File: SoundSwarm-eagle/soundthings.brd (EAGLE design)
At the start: 100 x 40 mm, 33 parts, among them Q2 IRLB8721PBF

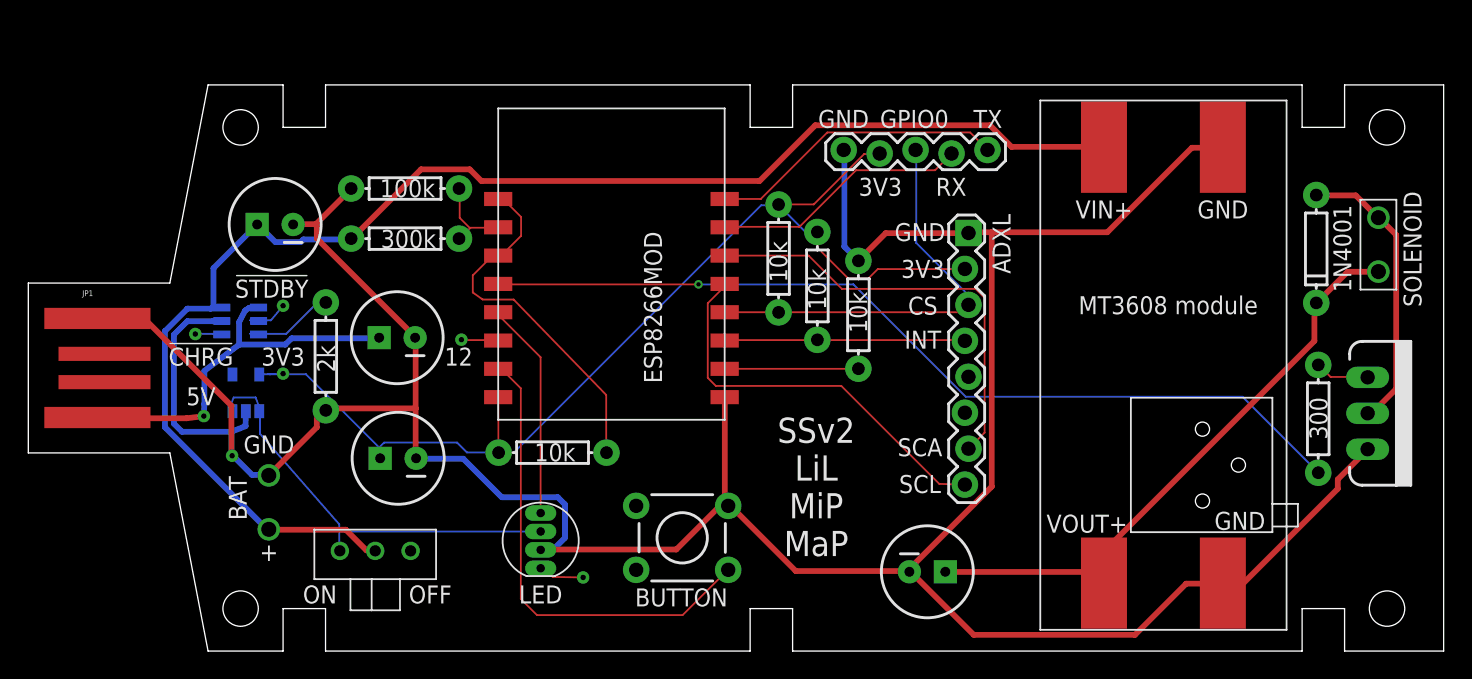
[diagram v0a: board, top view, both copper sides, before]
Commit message: As submitted to ditrypcbs
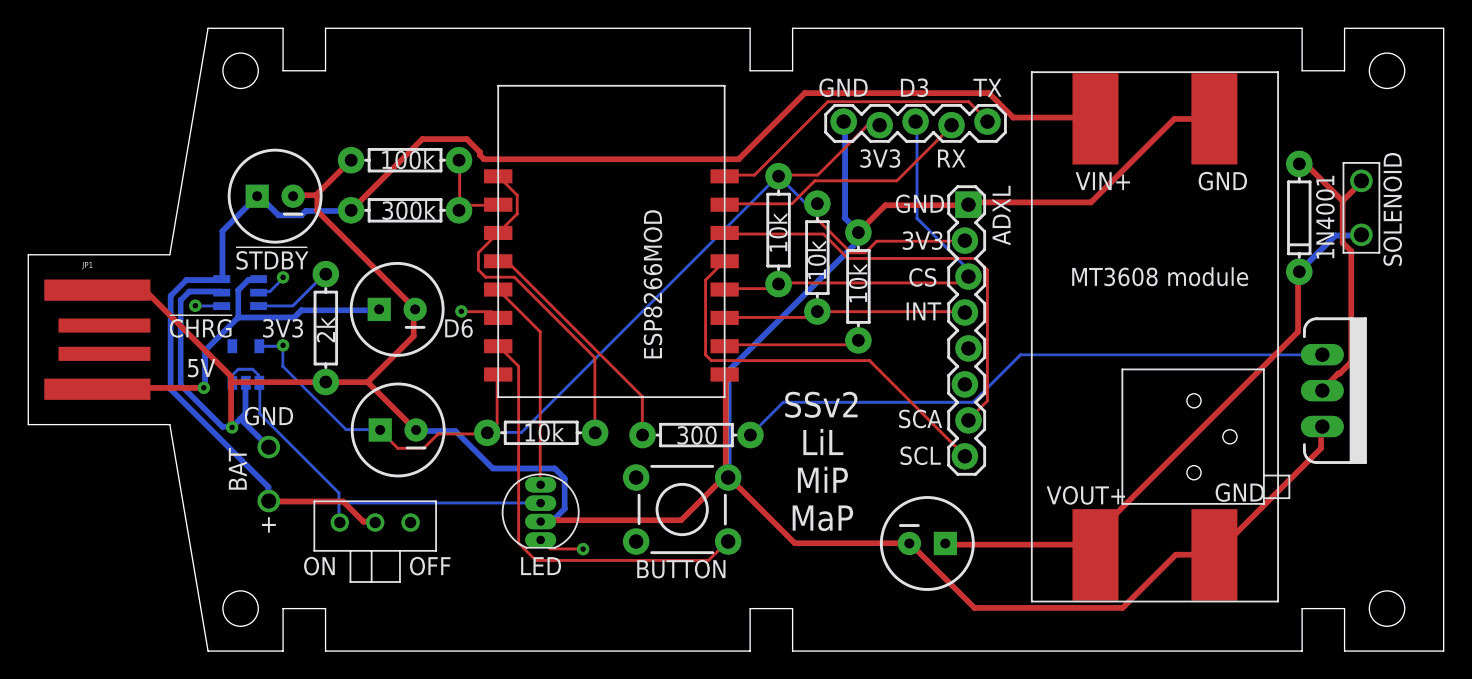
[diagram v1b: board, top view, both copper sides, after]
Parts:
- removed GPIO12: TEST-POINTTP_15TH_THRU, SparkFun-Passives:TP_15TH
- added D6: TEST-POINTTP_15TH_THRU, SparkFun-Passives:TP_15TH
- moved R8 43.9 mm to (47.2, 15.3), turned to 180 degrees
- moved Q2 3.58 mm to (91.4, 18.4)
- moved SOLENOID 2.86 mm to (94.2, 29.4)
- moved D1 2.51 mm to (89.8, 30.6)
- moved U$7 2.09 mm to (79.6, 22.2)
- moved L1 2.00 mm to (36.2, 9.80)
- moved !CHRG 2.00 mm to (11.8, 24.4)
- moved !STDBY 2.00 mm to (18.0, 26.4)
- moved 3V3 2.00 mm to (18.0, 21.6)
- moved 5V 2.00 mm to (12.4, 18.6)
- moved ADXL 2.00 mm to (66.3, 31.5)
- moved BAT 2.00 mm to (17.0, 10.6)
- moved BUTTON 2.00 mm to (46.2, 10.0)
- moved C1 2.00 mm to (63.5, 7.60)
- moved C2 2.00 mm to (26.1, 15.6)
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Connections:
- net DIN renamed GPIO14
- net GPIO12: now also D6.P$1; no longer GPIO12.P$1
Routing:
- net GPIO16: track 63.5 -> 16.9 mm, vias 1 -> 0
- net GATE: track 3.86 -> 42.8 mm
- net GND: track 233.1 -> 221.2 mm
- net GPIO13: track 33.8 -> 30.4 mm
- net EN: track 25.7 -> 24.4 mm
- net !STDBY: track 3.39 -> 2.21 mm
- net N$11: track 6.82 -> 5.68 mm
- net VBAT: track 102.7 -> 102.0 mm
- net 3.3V: track 78.9 -> 78.2 mm
- net VOUT+: track 43.4 -> 42.9 mm
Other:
- board size 100 x 40 mm -> 100 x 44 mm
- board text added: "D3"
- board text added: "D6"
- board text removed: "12"
- board text removed: "GPIO0"
